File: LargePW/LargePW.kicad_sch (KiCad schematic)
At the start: 38 parts, among them J1 Conn_01x02_Female, J10 Conn_01x02_Female, J11 Conn_01x02_Female, J12 Conn_01x02_Female, J13 Conn_01x02_Female, J2 Conn_01x02_Female, J3 Conn_01x02_Female, J4 Conn_01x02_Female, J5 Conn_01x02_Female, J6 Conn_01x02_Female, J7 Conn_01x02_Female, J8 Conn_01x02_Female, J9 Conn_01x02_Female, K1 RAYEX-L90, Q1 TJ60S04M3L, Q2 TJ60S04M3L, Q3 TJ60S04M3L, Q4 TJ60S04M3L, Q5 BSS138, SW1 SW_SPST

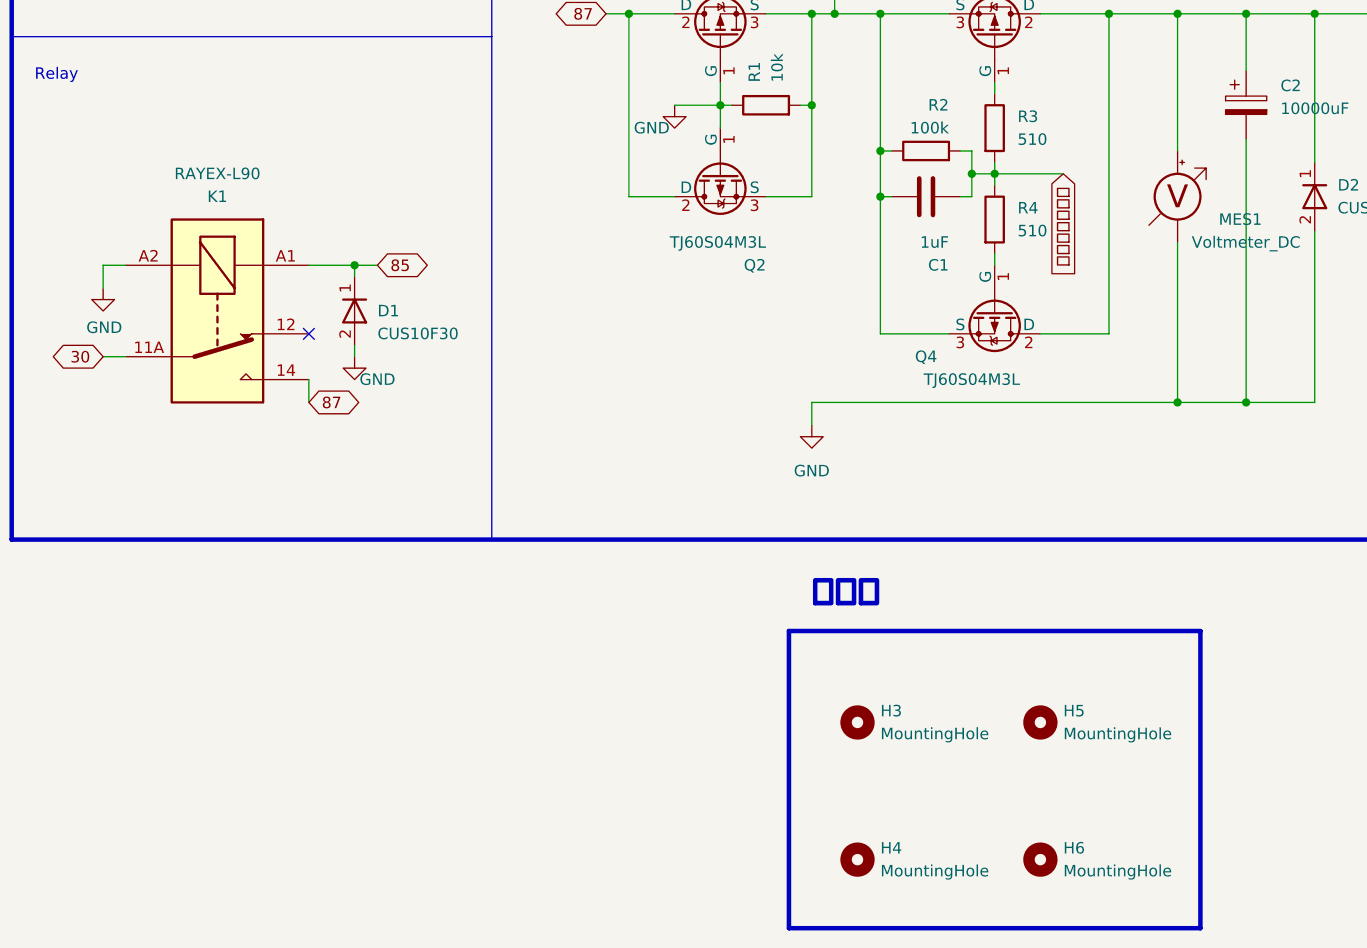
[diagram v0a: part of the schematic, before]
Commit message: SmallMDほぼ完成
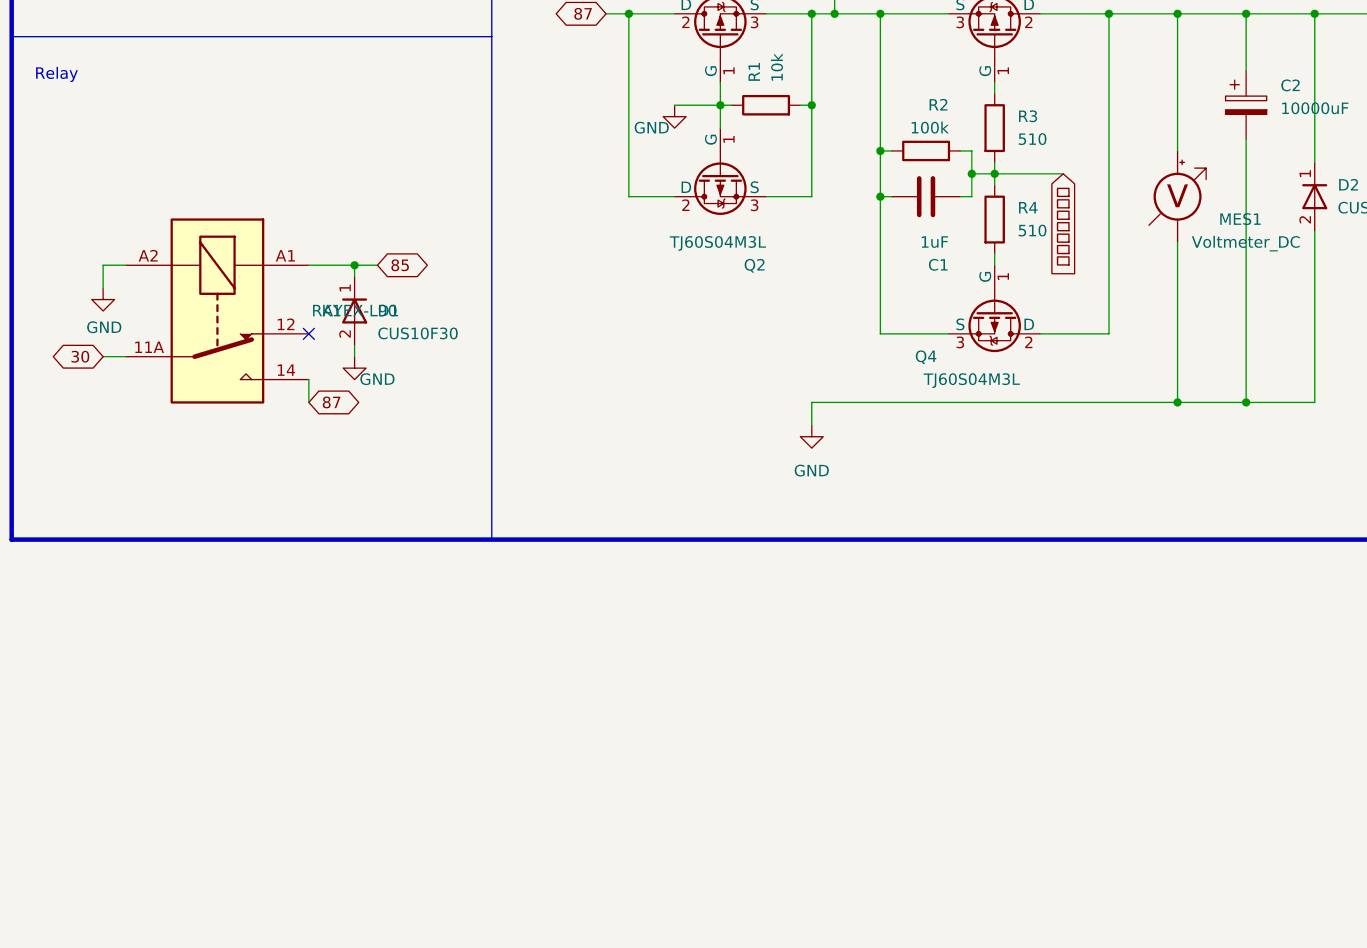
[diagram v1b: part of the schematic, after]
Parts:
- removed H3, H4, H5, H6: MountingHole, MountingHole:MountingHole_3.2mm_M3, symbol Mechanical:MountingHole
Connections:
- net 30: no longer K1.11B
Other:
- note removed: "ねじ穴"
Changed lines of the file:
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@@
     (stroke (width 0) (type default) (color 0 0 0 0))
-  )
-  (polyline (pts (xy 116.84 162.56) (xy 116.84 195.58))
-    (stroke (width 0.5) (type solid) (color 0 0 0 0))
   )
   (wire (pts (xy 238.76 104.14) (xy 236.22 104.14))
@@
   (wire (pts (xy 121.92 91.44) (xy 121.92 93.98))
     (stroke (width 0) (type default) (color 0 0 0 0))
-  )
-  (polyline (pts (xy 116.84 195.58) (xy 162.56 195.58))
-    (stroke (width 0.5) (type solid) (color 0 0 0 0))
   )
   (wire (pts (xy 162.56 48.26) (xy 165.1 48.26))
@@
     (stroke (width 0) (type default) (color 0 0 0 0))
   )
-  (polyline (pts (xy 162.56 195.58) (xy 162.56 162.56))
-    (stroke (width 0.5) (type solid) (color 0 0 0 0))
-  )
   (polyline (pts (xy 83.82 73.66) (xy 127 73.66))
     (stroke (width 0) (type default) (color 0 0 0 0))
@@
     (stroke (width 0) (type default) (color 0 0 0 0))
   )
-  (polyline (pts (xy 116.84 162.56) (xy 162.56 162.56))
-    (stroke (width 0.5) (type solid) (color 0 0 0 0))
-  )
   (wire (pts (xy 165.1 50.8) (xy 165.1 48.26))
     (stroke (width 0) (type default) (color 0 0 0 0))
@@
   (text "主電源スイッチ" (at 129.54 38.1 0)
     (effects (font (size 1.27 1.27)) (justify left bottom))
-  )
-  (text "ねじ穴" (at 119.38 160.02 0)
-    (effects (font (size 2.54 2.54) (thickness 0.508) bold) (justify left bottom))
   )
   (text "Fuse" (at 33.02 78.74 0)
@@
     (pin "2")
   )
-  (symbol (lib_id "Mechanical:MountingHole") (at 144.78 172.72 0) (unit 1)
-    (in_bom yes) (on_board yes) (fields_autoplaced)
-    (property "Reference" "H5" (id 0) (at 147.32 171.4499 0)
-      (effects (font (size 1.27 1.27)) (justify left))
-    )
-    (property "Value" "MountingHole" (id 1) (at 147.32 173.9899 0)
-      (effects (font (size 1.27 1.27)) (justify left))
-    )
-    (property "Footprint" "MountingHole:MountingHole_3.2mm_M3" (id 2) (at 144.78 172.72 0)
-      (effects (font (size 1.27 1.27)) hide)
-    )
-    (property "Datasheet" "~" (id 3) (at 144.78 172.72 0)
-      (effects (font (size 1.27 1.27)) hide)
-    )
-  )
   (symbol (lib_id "Connector:Conn_01x02_Female") (at 218.44 121.92 0) (unit 1)
     (in_bom yes) (on_board yes)
@@
     (pin "1")
   )
-  (symbol (lib_id "Mechanical:MountingHole") (at 124.46 187.96 0) (unit 1)
-    (in_bom yes) (on_board yes) (fields_autoplaced)
-    (property "Reference" "H4" (id 0) (at 127 186.6899 0)
-      (effects (font (size 1.27 1.27)) (justify left))
-    )
-    (property "Value" "MountingHole" (id 1) (at 127 189.2299 0)
-      (effects (font (size 1.27 1.27)) (justify left))
-    )
-    (property "Footprint" "MountingHole:MountingHole_3.2mm_M3" (id 2) (at 124.46 187.96 0)
-      (effects (font (size 1.27 1.27)) hide)
-    )
-    (property "Datasheet" "~" (id 3) (at 124.46 187.96 0)
-      (effects (font (size 1.27 1.27)) hide)
-    )
-  )
   (symbol (lib_id "Connector:Conn_01x02_Female") (at 243.84 139.7 0) (unit 1)
     (in_bom yes) (on_board yes)
@@
     )
     (pin "1")
-  )
-  (symbol (lib_id "Mechanical:MountingHole") (at 124.46 172.72 0) (unit 1)
-    (in_bom yes) (on_board yes) (fields_autoplaced)
-    (property "Reference" "H3" (id 0) (at 127 171.4499 0)
-      (effects (font (size 1.27 1.27)) (justify left))
-    )
-    (property "Value" "MountingHole" (id 1) (at 127 173.9899 0)
-      (effects (font (size 1.27 1.27)) (justify left))
-    )
-    (property "Footprint" "MountingHole:MountingHole_3.2mm_M3" (id 2) (at 124.46 172.72 0)
-      (effects (font (size 1.27 1.27)) hide)
-    )
-    (property "Datasheet" "~" (id 3) (at 124.46 172.72 0)
-      (effects (font (size 1.27 1.27)) hide)
-    )
   )
   (symbol (lib_id "power:VDD") (at 182.88 91.44 0) (unit 1)
@@
     (pin "1")
   )
-  (symbol (lib_id "Mechanical:MountingHole") (at 144.78 187.96 0) (unit 1)
-    (in_bom yes) (on_board yes) (fields_autoplaced)
-    (property "Reference" "H6" (id 0) (at 147.32 186.6899 0)
-      (effects (font (size 1.27 1.27)) (justify left))
-    )
-    (property "Value" "MountingHole" (id 1) (at 147.32 189.2299 0)
-      (effects (font (size 1.27 1.27)) (justify left))
-    )
-    (property "Footprint" "MountingHole:MountingHole_3.2mm_M3" (id 2) (at 144.78 187.96 0)
-      (effects (font (size 1.27 1.27)) hide)
-    )
-    (property "Datasheet" "~" (id 3) (at 144.78 187.96 0)
-      (effects (font (size 1.27 1.27)) hide)
-    )
-  )
   (symbol (lib_id "Device:Q_PMOS_GDS") (at 139.7 127 270) (unit 1)
     (in_bom yes) (on_board yes)
@@
   (symbol (lib_id "Relay:RAYEX-L90") (at 53.34 127 270) (unit 1)
     (in_bom yes) (on_board yes)
-    (property "Reference" "K1" (id 0) (at 53.34 114.3 90))
-    (property "Value" "RAYEX-L90" (id 1) (at 53.34 111.76 90))
-    (property "Footprint" "Relay:TRV4-L-12V-Z-F" (id 2) (at 41.91 125.73 0)
+    (property "Reference" "K1" (id 0) (at 66.04 127 90))
+    (property "Value" "RAYEX-L90" (id 1) (at 68.58 127 90))
+    (property "Footprint" "Relay:TRV4-L-12V-Z-F" (id 2) (at 54.61 115.57 0)
       (effects (font (size 1.27 1.27)) (justify left) hide)
     )
-    (property "Datasheet" "https://a3.sofastcdn.com/attachment/7jioKBjnRiiSrjrjknRiwS77gwbf3zmp/L90-SERIES.pdf" (id 3) (at 44.45 152.4 0)
+    (property "Datasheet" "https://a3.sofastcdn.com/attachment/7jioKBjnRiiSrjrjknRiwS77gwbf3zmp/L90-SERIES.pdf" (id 3) (at 27.94 118.11 0)
       (effects (font (size 1.27 1.27)) (justify left) hide)
     )
     (pin "11A")
-    (pin "11B")
     (pin "12")
     (pin "14")
@@
       (reference "H2") (unit 1) (value "MountingHole_Pad") (footprint "TestPoint:TestPoint_THTPad_D4.0mm_Drill2.0mm")
     )
-    (path "/94f2f40a-5d3e-4e2a-827f-1631827b1839"
-      (reference "H3") (unit 1) (value "MountingHole") (footprint "MountingHole:MountingHole_3.2mm_M3")
-    )
-    (path "/81bf1c9c-4f8f-48e0-84bb-2d762d2317c8"
-      (reference "H4") (unit 1) (value "MountingHole") (footprint "MountingHole:MountingHole_3.2mm_M3")
-    )
-    (path "/3fe896f8-123e-4baa-8564-2a9ea447d311"
-      (reference "H5") (unit 1) (value "MountingHole") (footprint "MountingHole:MountingHole_3.2mm_M3")
-    )
-    (path "/d4545894-3a7e-48f8-a806-498d5ab658af"
-      (reference "H6") (unit 1) (value "MountingHole") (footprint "MountingHole:MountingHole_3.2mm_M3")
-    )
     (path "/e80e9d3f-5cdd-4bd1-847e-d26e89dd98ef"

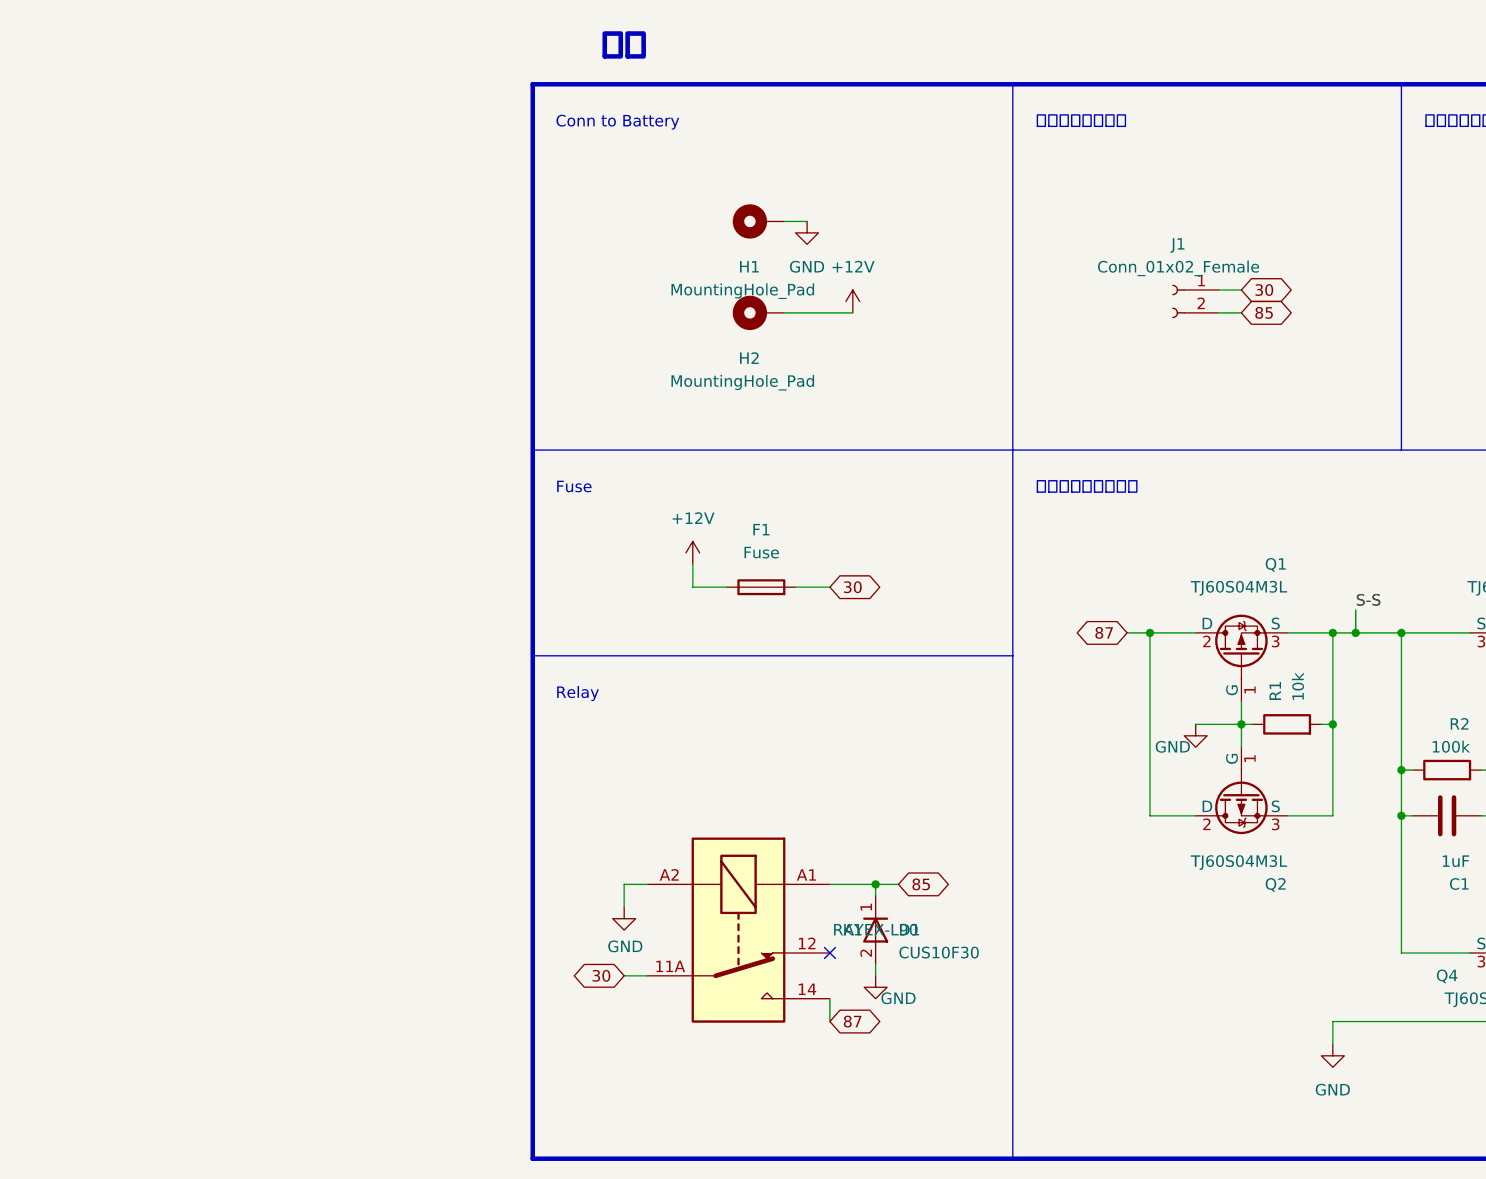
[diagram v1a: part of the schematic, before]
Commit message: 製造ファイル出力その2
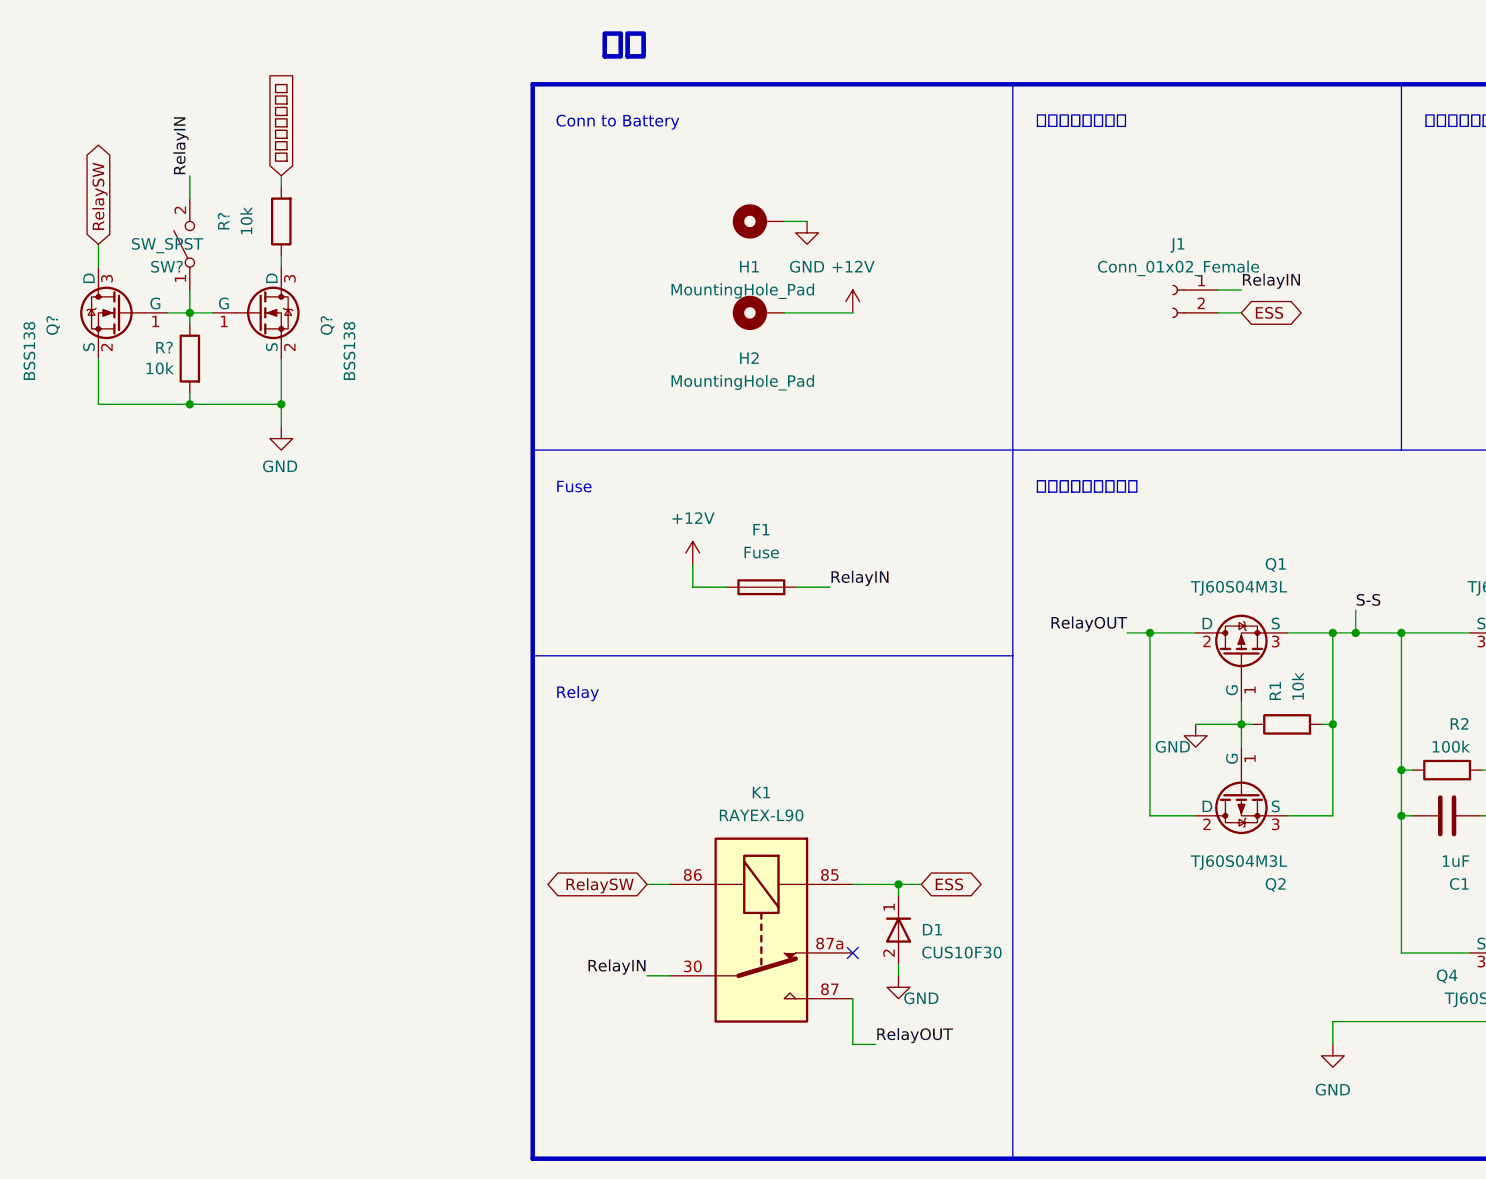
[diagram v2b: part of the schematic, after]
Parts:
- added Q? (x2): BSS138, Package_TO_SOT_SMD:SOT-23_Handsoldering, symbol Device:Q_NMOS_GSD
- added R? (x2): 10k, Resistor_SMD:R_0603_1608Metric_Pad0.98x0.95mm_HandSolder, symbol Device:R
- added SW?: SW_SPST, Rocker_Switch:DS-850K-S-ON, symbol Switch:SW_SPST
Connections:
- net GND: now also Q?.2 (S), Q?.2 (S), R?.2; no longer K1.A2
- net 主電源スイッチ: now also R?.2
- net 30 renamed RelayIN
- net RelayIN: now also K1.30, SW?.2 (B); no longer K1.11A
- net 85 renamed ESS
- net ESS: now also K1.85; no longer K1.A1
- net 87 renamed RelayOUT
- net RelayOUT: now also K1.87; no longer K1.14
- new net: Q?.3 (D), R?.1
- new net: Q?.1 (G), Q?.1 (G), R?.1, SW?.1 (A)
- new net RelaySW: K1.86, Q?.3 (D)
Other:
- moved on the sheet: D1, K1
